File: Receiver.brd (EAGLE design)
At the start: 71.1 x 62.2 mm, 11 parts, among them IC1 25LC080P, J1 PIC_ICSP_6_PIN, U1 915MHz, U2 DS3234, X1 BU-SMA-V

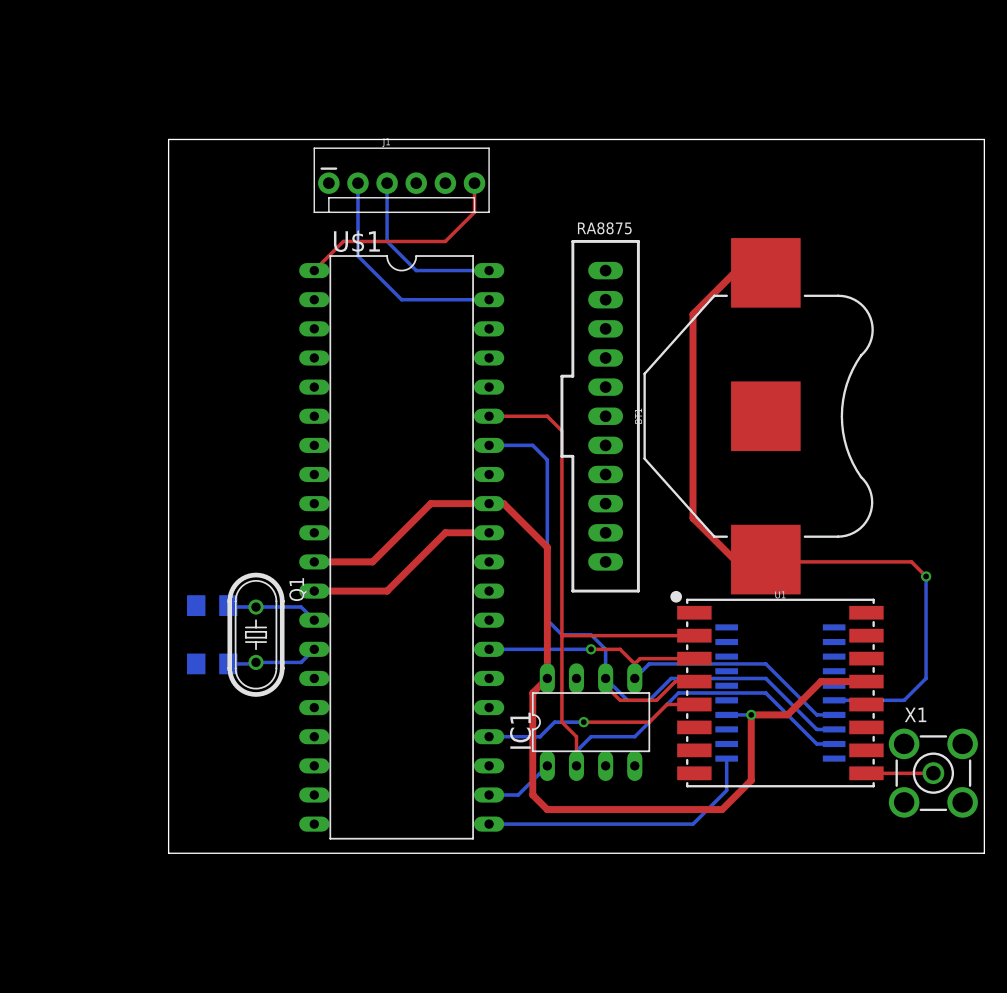
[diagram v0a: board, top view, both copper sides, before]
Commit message: Updates
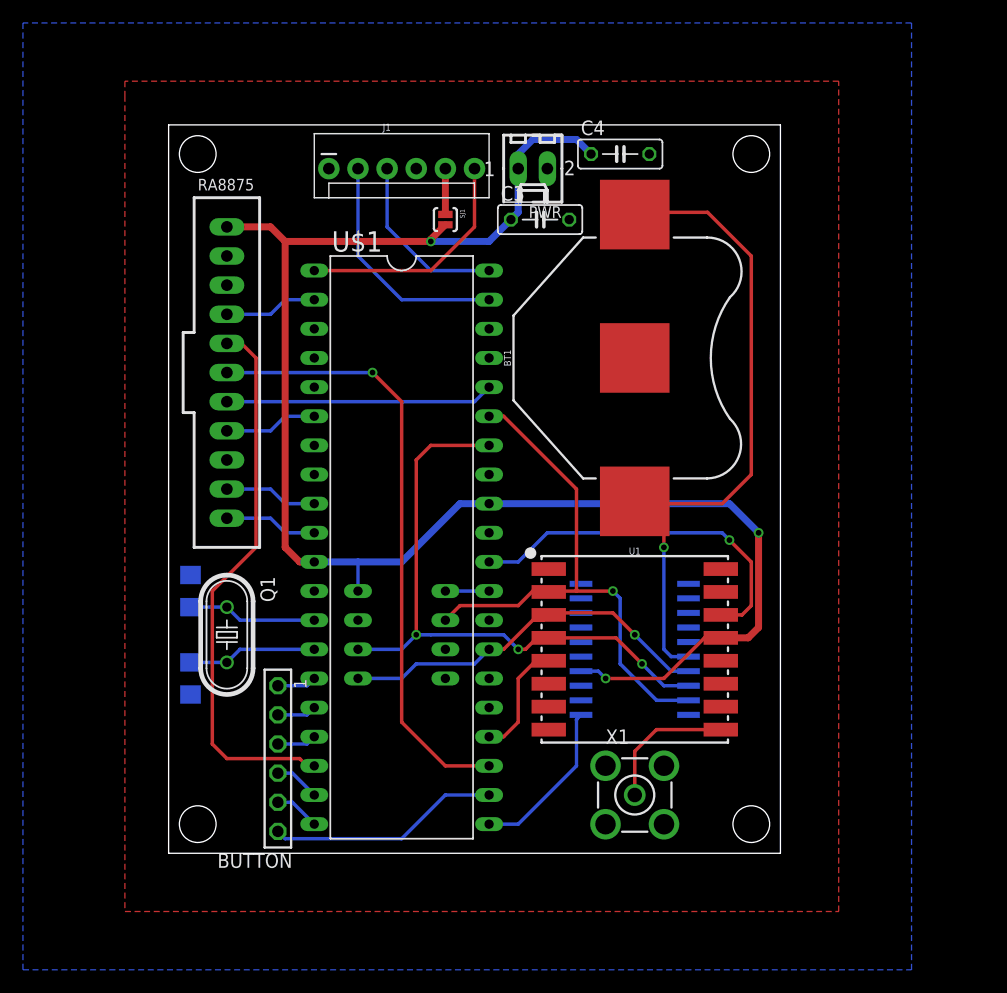
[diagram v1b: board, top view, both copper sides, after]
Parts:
- added BUTTON: TSW-106-02-S-S, con-samtec:TSW-106-02-S-S
- added C3, C4: (no value), resistor:C050-025X075
- added PWR: 22-27-2021-02, con-molex:6410-02
- added SJ1: SOLDERJUMPERNO, SparkFun-Retired:SJ_2S-NO
- moved RA8875 33.2 mm to (5.08, 41.9)
- moved X1 26.1 mm to (40.6, 5.08)
- moved IC1 18.2 mm to (20.3, 19.1), flipped to the bottom, turned to 270 degrees
- moved U1 13.3 mm to (40.6, 17.8)
- moved U2 13.3 mm to (40.6, 17.8)
- moved BT1 12.5 mm to (40.6, 43.2)
- moved Q1 2.54 mm to (5.08, 19.1)
- moved C1 2.29 mm to (1.91, 15.2), turned to 90 degrees
- moved C2 2.29 mm to (1.91, 22.9), turned to 270 degrees
- moved J1 1.27 mm to (14.0, 59.7)
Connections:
- net N$10 renamed MOSI1
- net N$11 renamed MOSI2
- net N$6 renamed SCK1
- net N$7 renamed MISO1
- net N$8 renamed SCK2
- net N$9 renamed MISO2
- new net N$10: BUTTON.4, U$1.19
- new net N$11: BUTTON.6, U$1.22
- new net N$17: RA8875.8, U$1.6
- new net N$18: RA8875.4, U$1.2
- new net N$19: RA8875.10, U$1.9
- new net N$20: RA8875.11, U$1.10
- new net N$21: U$1.30, U1.14
- new net N$22: J1.5, SJ1.1
- new net N$6: BUTTON.1, U$1.15
- new net N$7: BUTTON.2, U$1.16
- new net N$8: BUTTON.3, U$1.17
- new net N$9: BUTTON.5, U$1.20
- net +3V3: now also C3.1, C4.1, PWR.1, RA8875.1, SJ1.2; no longer J1.5
- net GND: now also C3.2, C4.2, PWR.2
- net N$12: now also U$1.29; no longer U$1.22
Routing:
- net +3V3: track 85.8 -> 141.4 mm, vias 1 -> 3
- net MISO1: track 0.00 -> 53.4 mm, vias 0 -> 1
- net SCK1: track 0.00 -> 48.0 mm
- net N$21: track 0.00 -> 31.8 mm, vias 0 -> 1
- net MISO2: track 75.8 -> 48.7 mm, vias 0 -> 1
- net MOSI1: track 0.00 -> 23.4 mm
- net N$11: track 0.00 -> 20.3 mm
- net GND: track 17.3 -> 0.00 mm
- net N$16: track 24.7 -> 14.3 mm
- net N$15: track 19.1 -> 10.2 mm, vias 1 -> 0
- net N$17: track 0.00 -> 8.15 mm
- net N$20: track 0.00 -> 8.15 mm
- net N$19: track 0.00 -> 8.15 mm
- net N$18: track 0.00 -> 8.15 mm
- net N$14: track 65.7 -> 58.2 mm
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- added copper zone on layer 1, net GND
- added copper zone on layer 16, net GND
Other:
- board size 71.1 x 62.2 mm -> 53.3 x 63.5 mm
